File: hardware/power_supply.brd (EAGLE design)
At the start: 76.2 x 38.1 mm, 29 parts, among them Q1 IRF630N, U1 MC34063

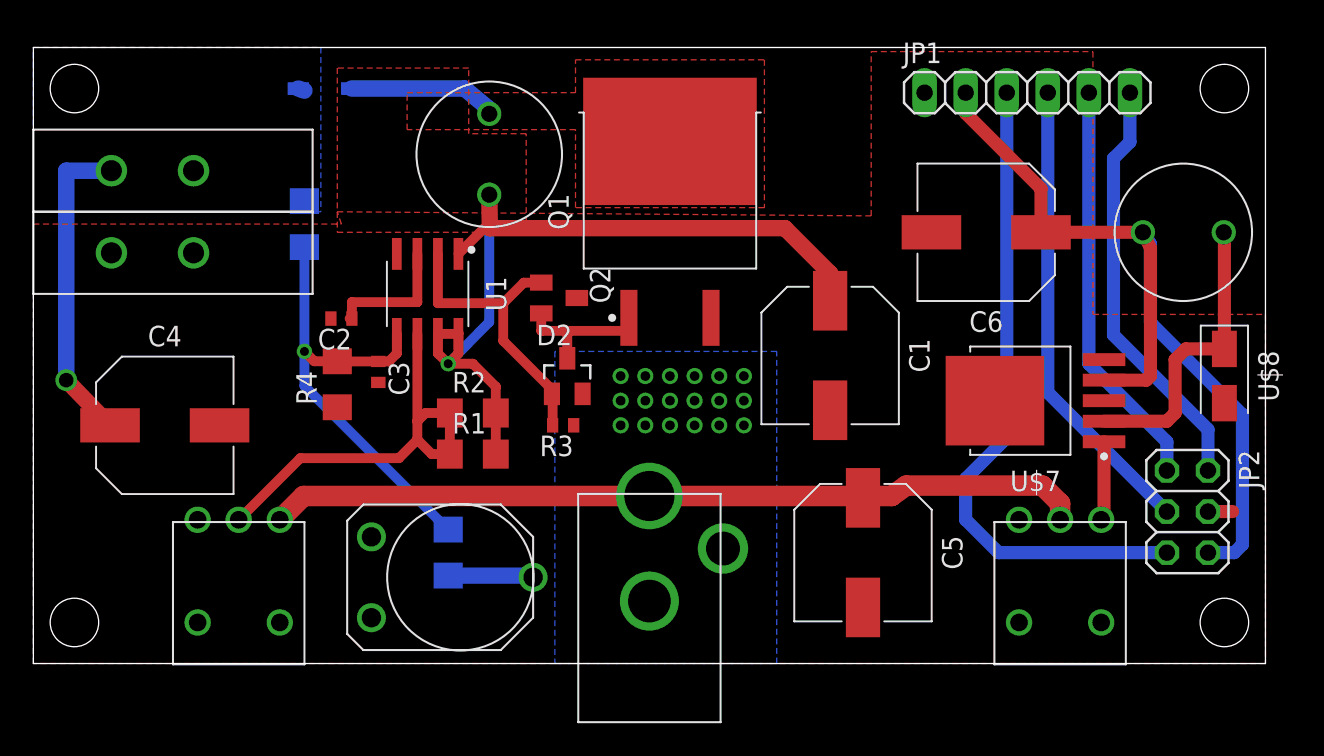
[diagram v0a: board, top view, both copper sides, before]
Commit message: Updating power supply 7/10
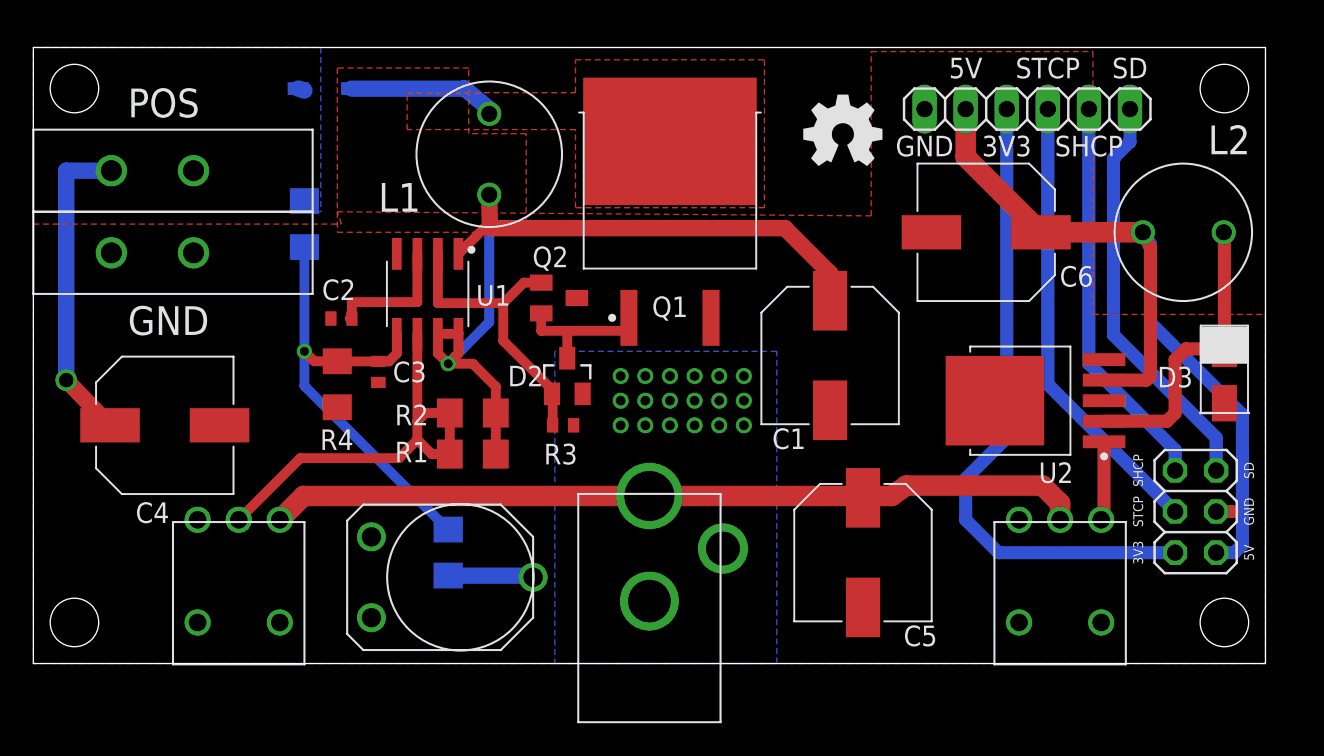
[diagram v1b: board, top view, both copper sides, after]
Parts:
- moved JP1 1.02 mm to (61.5, 34.3)
- moved JP2 0.51 mm to (71.9, 9.40)
- renumbered U$7 to U2, U$8 to D3
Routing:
- net +5V: track 53.0 -> 51.5 mm
- net STCP: track 29.0 -> 28.2 mm
- net SHCP: track 25.4 -> 24.6 mm
- net DI: track 26.2 -> 25.4 mm
- net +3V3: track 40.8 -> 40.2 mm
- net GND: track 1.52 -> 1.02 mm
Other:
- board text added: "3V3"
- board text added: "5V"
- board text added: "GND"
- board text added: "L1"
- board text added: "L2"
- board text added: "POS"
- board text added: "SD"
- board text added: "SHCP"
- board text added: "STCP"
- board text added: "https://github.com/bmboucher/nixie_ticker"
